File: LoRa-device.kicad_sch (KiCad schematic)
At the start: 141 parts, among them J1 Micro_SD_Card_Det1, J2 Conn_01x02_Pin, J3 Conn_01x04_Pin, J4 Conn_01x14_Pin, J6 Conn_01x04_Pin, J8 U.FL, SW2 SW_DPST_x2, U1 ESP32-S3, U10 TPS2116DRL, U11 MC-121-L119, U12 K2-1102AQ-K4CW-01, U13 MCP23S17_ML, U14 MAX98357A, U15 HJ-SMA275, U16 Black_headphone_jack, U17 RA-01SH-P, U18 L76KB-A58, U19 TF-01A, U2 W25Q128JVS, U20 MAX98357AETE+T, U3 TP4055, U4 STLQ015M33R, U5 Ai-Thinker-Ra-01, U6 USBLC6-2P6, U7 K2-1102AQ-K4CW-01, U8 TPS22917LDBV, U9 AP63203WU, Y1 32.768 kHz, Y2 40MHz(10ppm)

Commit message: To be routed, most work likely done.
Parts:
- removed R1, R4: 10K, Resistor_SMD:R_0402_1005Metric, symbol Device:R
- removed R24: 470R, Resistor_SMD:R_0402_1005Metric, symbol Device:R
- removed R41, R42: 4.7kΩ, PCM_JLCPCB:R_0402, symbol PCM_JLCPCB-Resistors:0402,4.7kΩ
- removed SW2: SW_DPST_x2, Connector_PinHeader_2.54mm:PinHeader_1x02_P2.54mm_Vertical, symbol Switch:SW_DPST_x2
- removed U13: MCP23S17_ML, Package_DFN_QFN:QFN-28-1EP_6x6mm_P0.65mm_EP4.25x4.25mm, symbol Interface_Expansion:MCP23S17_ML
- removed U14: MAX98357A, Package_DFN_QFN:TQFN-16-1EP_3x3mm_P0.5mm_EP1.23x1.23mm, symbol Audio:MAX98357A
- removed U19: TF-01A, LoRa_library:TF-SMD_TF-01A, symbol LoRa_library:TF-01A
- removed U20: MAX98357AETE+T, LoRa_library:TQFN-16_L3.0-W3.0-P0.50-BL-EP1.5, symbol LoRa_library:MAX98357AETE+T
- removed U5: Ai-Thinker-Ra-01, RF_Module:Ai-Thinker-Ra-01-LoRa, symbol RF_Module:Ai-Thinker-Ra-01
- added R24, R42: 330Ω, PCM_JLCPCB:R_0402, symbol PCM_JLCPCB-Resistors:0402,330Ω
- added R4: 10kΩ, PCM_JLCPCB:R_0402, symbol PCM_JLCPCB-Resistors:0402,10kΩ
- added R44, R45, R46: 33Ω, PCM_JLCPCB:R_0402, symbol PCM_JLCPCB-Resistors:0402,33Ω
- added R47, R48: 2.2kΩ, PCM_JLCPCB:R_0402, symbol PCM_JLCPCB-Resistors:0402,2.2kΩ
- added U14: MCP23017_ML, Package_DFN_QFN:QFN-28-1EP_6x6mm_P0.65mm_EP4.25x4.25mm, symbol Interface_Expansion:MCP23017_ML
- added U19: MAX98357A, Package_DFN_QFN:TQFN-16-1EP_3x3mm_P0.5mm_EP1.23x1.23mm, symbol Audio:MAX98357A
- added U5: SK-12D02-VG5, LoRa_library:SW-TH_SK-12D02-VG5, symbol LoRa_library:SK-12D02-VG5
- J2: footprint Connector_PinHeader_2.54mm:PinHeader_1x02_P2.54mm_Vertical -> Connector_PinHeader_1.27mm:PinHeader_1x02_P1.27mm_Vertical
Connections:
- net LORA_IO0 is gone; now on net SCREEN_CS: U1.7 (GPIO2)
- net +3V3: now also U17.3 (3V3), R4.1, R47.1, R48.1, U14.5 (VDD), U19.7 (VDD), U19.8 (VDD)
- net GND: now also J1.11 (SHIELD), J1.12 (SHIELD), J1.13 (SHIELD), J8.3 (Ext), U17.16 (GND), U17.17 (GND), U17.2 (GND), U17.9 (GND), U14.11 (A0), U14.12 (A1), U14.13 (A2), U14.29 (EP), U14.6 (VSS), U19.11 (GND), U19.15 (GND), U19.17 (PAD), U19.3 (GND), U5.2, U5.4, U5.5
- net GPA5: now also U14.22 (GPA5)
- net GPA6: now also U14.23 (GPA6)
- net GPB6: now also U14.3 (GPB6)
- net GPB7: now also U14.4 (GPB7)
- net GPS_1PPS: now also U14.28 (GPB3); no longer U1.12 (GPIO7)
- net GPS_RST: now also U14.20 (GPA3)
- net GPS_WKUP: now also U14.21 (GPA4)
- net IO1: now also U19.14 (LRCLK)
- net IO10: now also U14.16 (INTA)
- net IO18: now also U14.15 (INTB)
- net IO4: now also U19.16 (BCLK)
- net LORA_IO1: now also R44.1, U14.18 (GPA1)
- net LORA_IO2: now also R45.1, U14.25 (GPB0)
- net LORA_IO3: now also R46.1, U14.26 (GPB1)
- net LORA_RST: now also U17.4 (RESET), U14.17 (GPA0)
- net MISOA: now also U17.13 (MISO)
- net MOSIA: now also U17.14 (MOSI)
- net SCKA: now also U17.12 (SCK)
- net SCREEN_LED: now also U1.16 (GPIO11); no longer U1.14 (GPIO9)
- net SCREEN_RST: now also U14.19 (GPA2)
- net SD_CS: now also U1.23 (GPIO17)
- net SPICLK_N/IO48/LORA_CS: now also U17.15 (NSS)
- net TOUCH_CS: now also U1.11 (GPIO6)
- net TOUCH_IRQ: now also U14.1 (GPB4); no longer U1.11 (GPIO6)
- net at U1.49 (U0TXD): now also R42.1
- net at R7.1, U8.3 (~{ON}): now also U5.3
- net at R38.2: now also U19.4 (~{SD_MODE})
- net at DNP2.1, L1.1: now also U17.1 (ANT)
- net at R5.2: now also U19.1 (DIN)
- net LORA_BUSY: now reaches U17.10 (BUSY)
- net LORA_BUSY: now also U1.12 (GPIO7)
- net LORA_RF_EN: now reaches U17.11 (RF_EN)
- net LORA_RF_EN: now also U14.27 (GPB2)
- net at U17.6 (DIO1): now also R44.2
- net at U17.7 (DIO2): now also R45.2
- net at U17.8 (DIO3): now also R46.2
- net at U16.3 (GND): now also U19.10 (OUTN)
- net at JP3.2 (C): now also U19.2 (GAIN_SLOT)
- net at U16.4 (L): now also U19.9 (OUTP)
- net IO11/BAT renamed IO9/BAT
- net IO9/BAT: now also U1.14 (GPIO9); no longer U1.16 (GPIO11)
- net IO17 renamed GPA7
- net GPA7: now also U14.24 (GPA7); no longer U1.23 (GPIO17)
- net SPICLK_P/IO47/EXP_CS renamed SPICLK_P/IO47/EXP_RST
- net SPICLK_P/IO47/EXP_RST: now also R4.2, U14.14 (~{RESET})
- net U0RXD/IO44: no longer names the net of U1.50 (U0RXD)
- net U0RXD/IO44: now also R24.1; no longer J3.2 (Pin_2)
- net U0TXD/IO43 renamed U0TXD/IO43/I2C_SCK
- net U0TXD/IO43/I2C_SCK: now also R42.2, R48.2, U14.8 (SCK)
- new net U0RXD/IO44/I2C_SDA: J3.2 (Pin_2), R24.2, R47.2, U14.9 (SDA)
- no-connect marks 22 -> 25
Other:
- moved on the sheet: C36, C44, C45, C7, DNP2, DNP4, J3, L1, R10, R22, U15

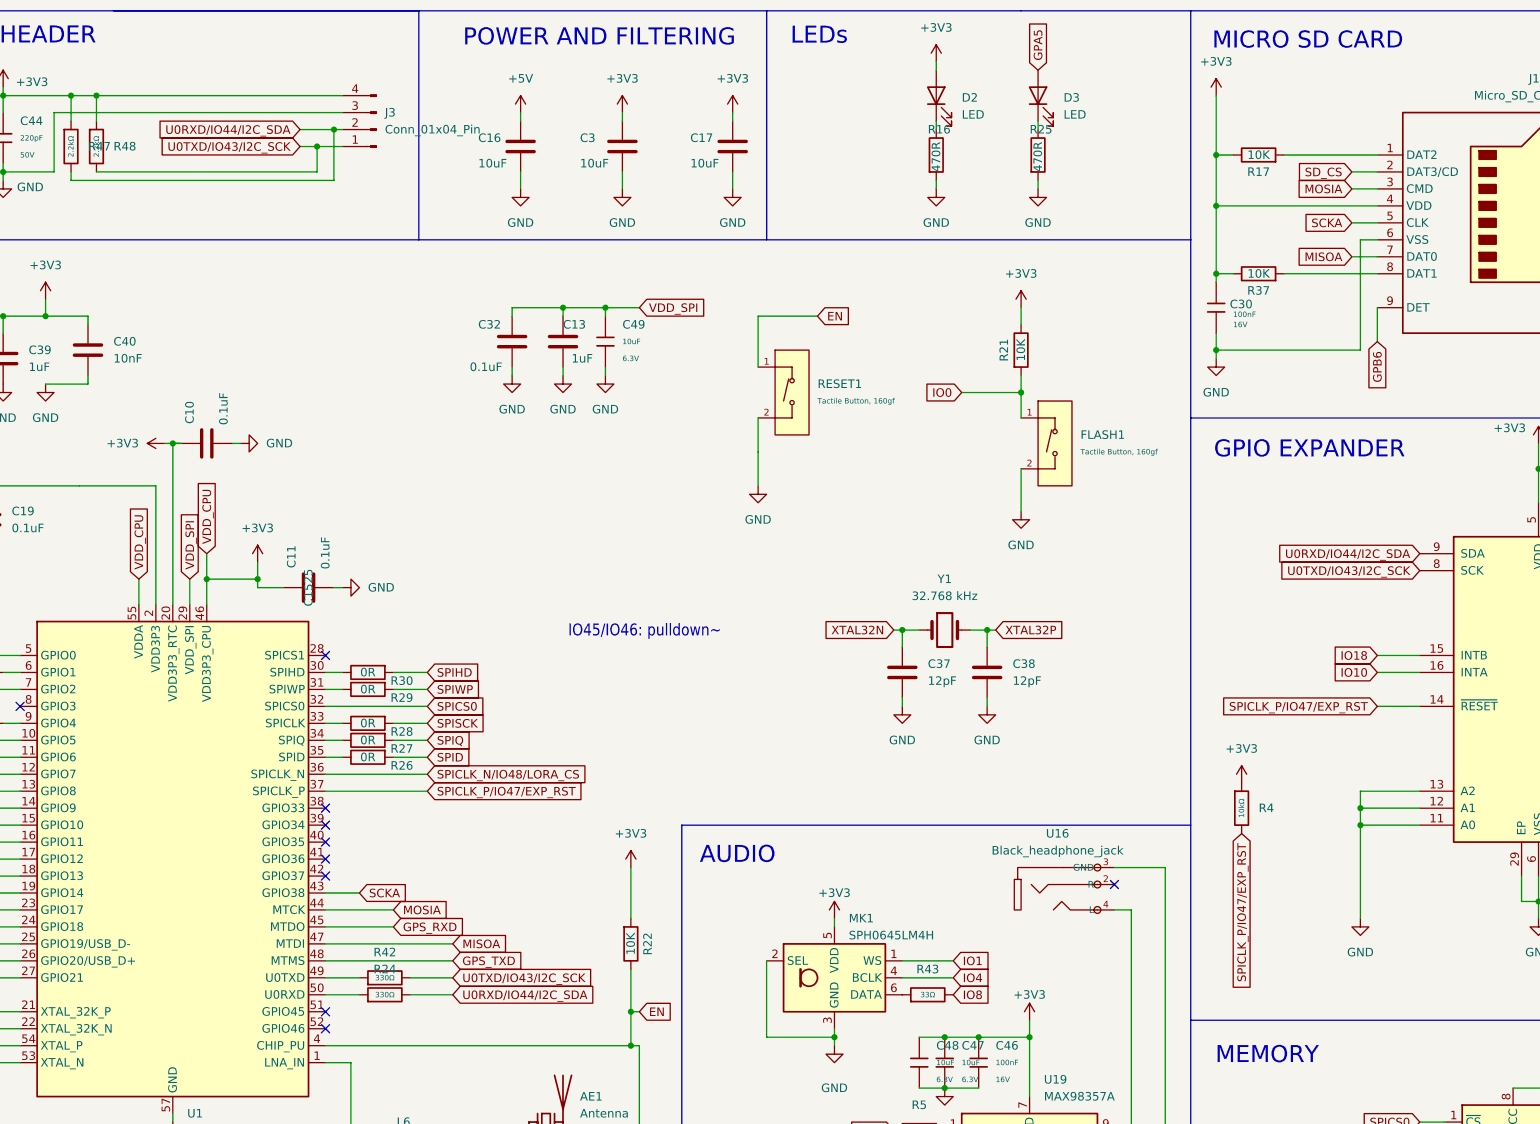
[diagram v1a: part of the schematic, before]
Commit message: new case design.
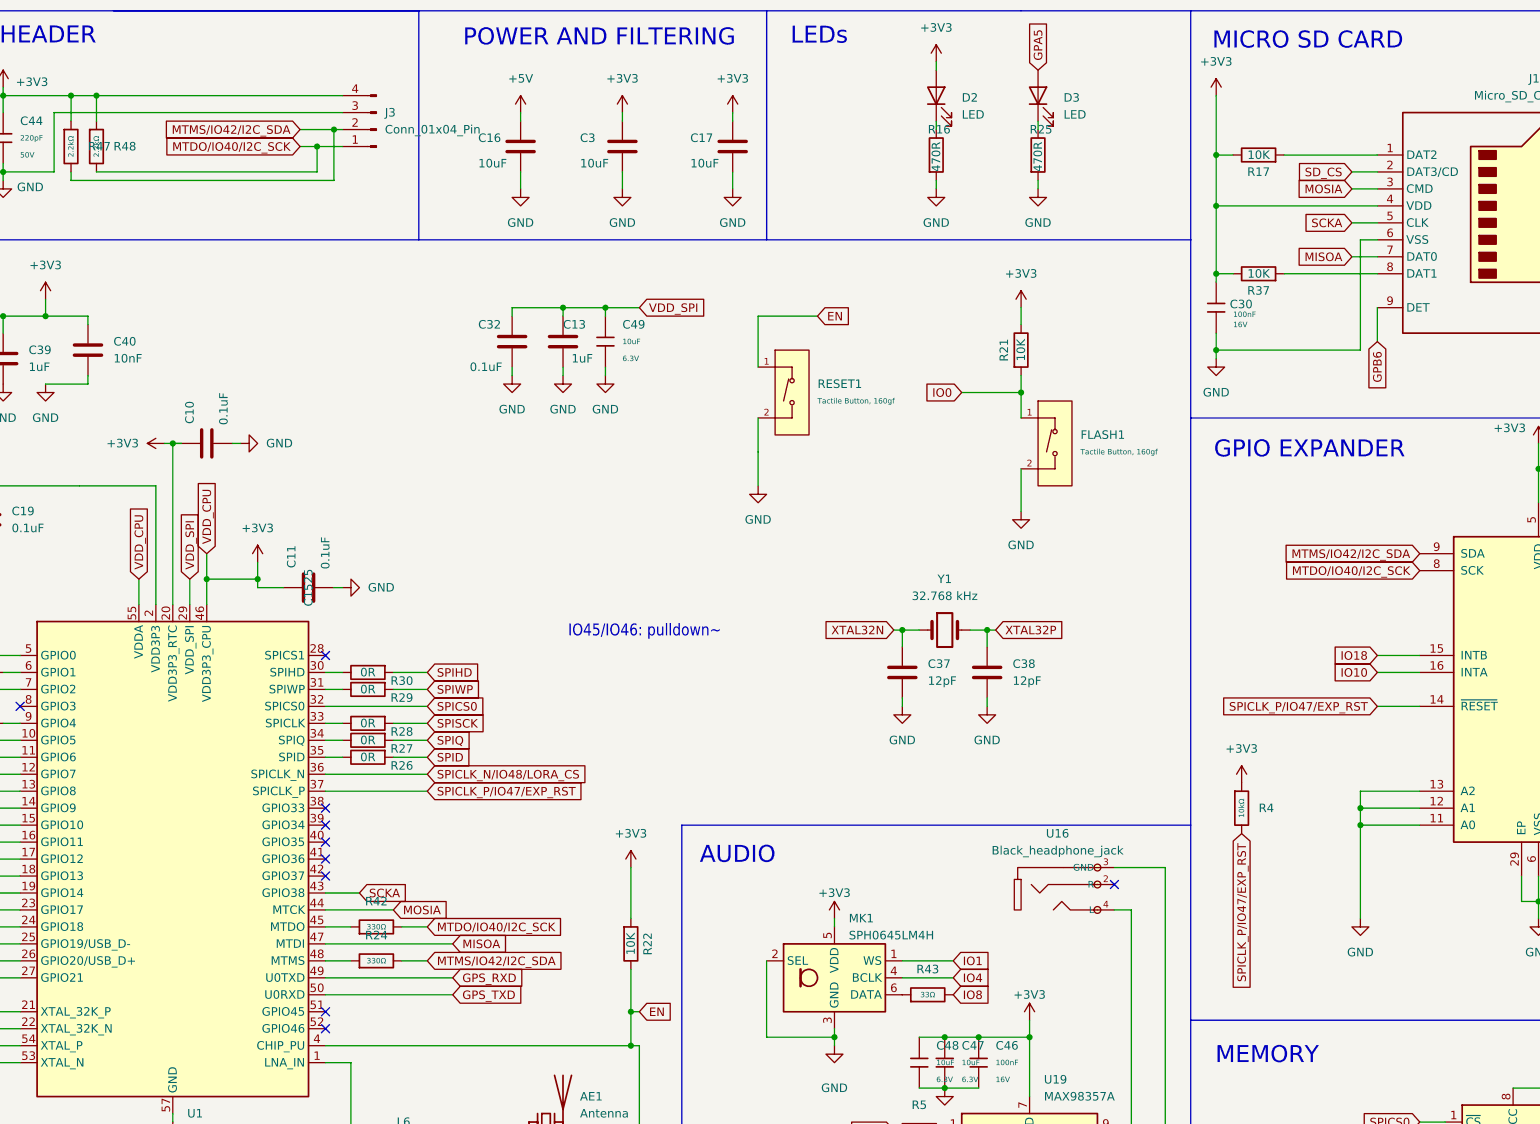
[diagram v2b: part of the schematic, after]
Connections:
- net GPS_RXD: now also U1.49 (U0TXD); no longer U1.45 (MTDO)
- net GPS_TXD: now also U1.50 (U0RXD); no longer U1.48 (MTMS)
- net at R24.1: now also U1.48 (MTMS); no longer U1.50 (U0RXD)
- net at R42.1: now also U1.45 (MTDO); no longer U1.49 (U0TXD)
- net U0RXD/IO44/I2C_SDA renamed MTMS/IO42/I2C_SDA
- net U0TXD/IO43/I2C_SCK renamed MTDO/IO40/I2C_SCK
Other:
- moved on the sheet: R24, R42
